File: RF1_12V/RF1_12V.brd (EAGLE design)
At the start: 6.9 x 7.1 mm, 17 parts, among them IC1 L78L33ACZ, IC2 MCP1702, J1 12V, Q1 16mhz, U1 ATMEGA328P_PDIP

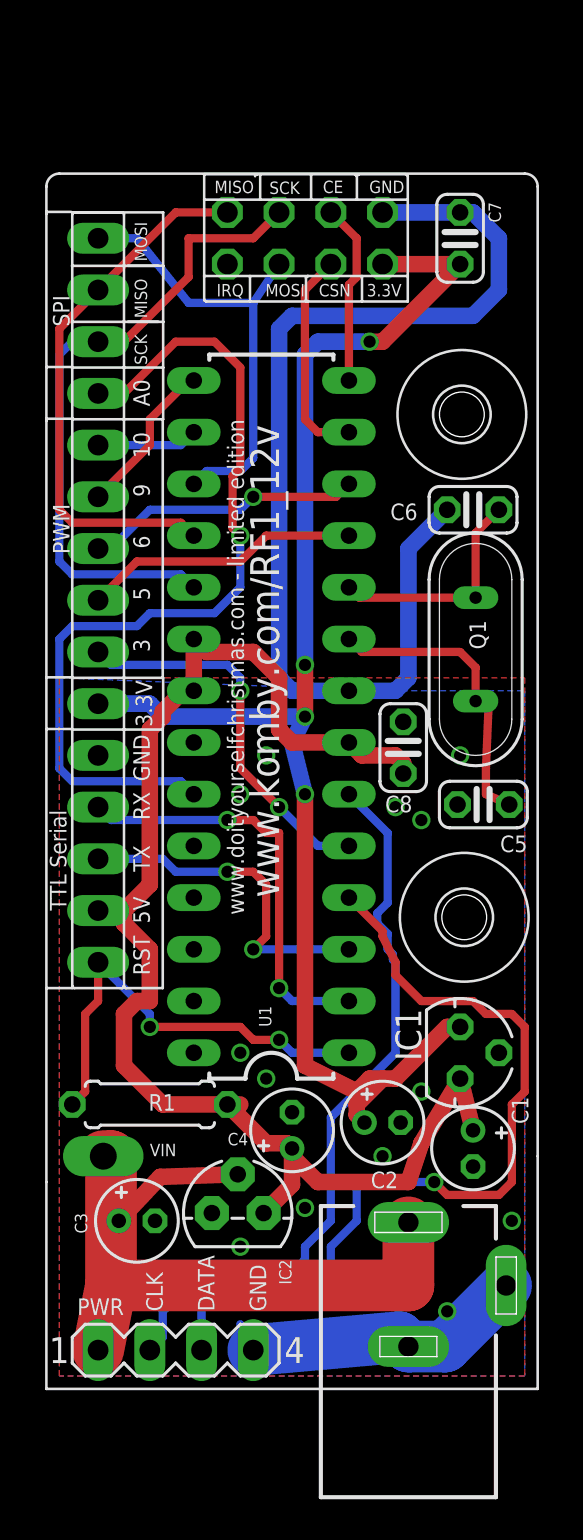
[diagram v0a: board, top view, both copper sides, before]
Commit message: Updated with 2014 designs for both RF1_12v and RF1 5v
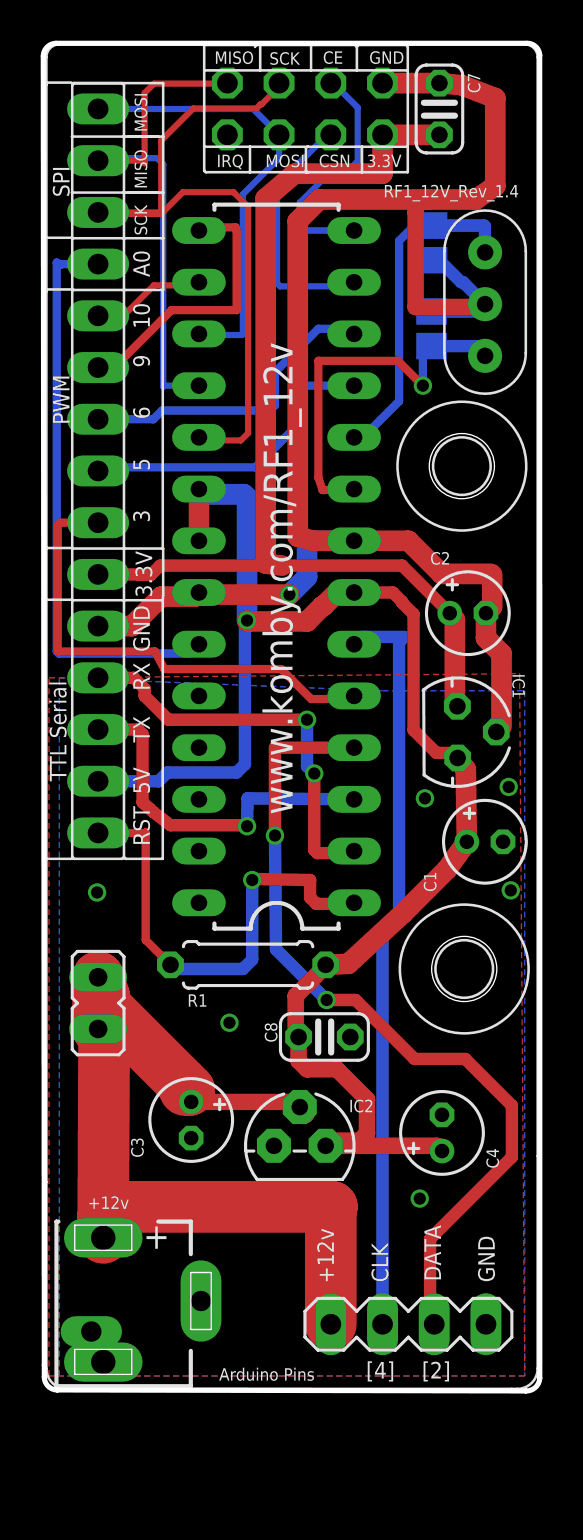
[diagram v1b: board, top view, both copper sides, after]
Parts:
- removed Q1: 16mhz, special:QS
- removed TP1: PTR1PAD1-13Y, testpad:P1-13Y
- added JP1: +12v, jumper:JP1
- added U$2: (no value), adafruit:CERM_OSC
- C2: value .1uf -> .1uF
- C3, C4: value 1uF -> 10uF
- C5, C6: device resistor:C025-024X044 -> adafruit:C0805
- C7, C8: value 100n -> .1uF
- J1: device con-jack:DCJ0303 -> con-jack_komby:DCJ0303
- moved C2 25.4 mm to (20.7, 38.1)
- moved C5 23.5 mm to (18.9, 52.1), flipped to the bottom, turned to 90 degrees
- moved IC1 15.7 mm to (20.2, 32.3), turned to 270.3 degrees
- moved C1 15.1 mm to (21.5, 26.9), turned to 0 degrees
- moved J1 15.0 mm to (2.79, 4.32)
- moved C8 14.7 mm to (13.7, 17.3), turned to 0 degrees
- moved C6 13.3 mm to (18.9, 56.3), flipped to the bottom, turned to 270 degrees
- moved SV1 11.5 mm to (17.8, 3.17)
- moved R1 8.39 mm to (9.91, 20.8)
- moved U1 7.37 mm to (11.3, 40.4)
- moved C4 7.37 mm to (19.4, 12.6)
- moved C7 6.43 mm to (19.3, 62.9)
- moved C3 5.63 mm to (7.11, 13.2), turned to 270 degrees
- moved IC2 4.49 mm to (12.4, 11.9)
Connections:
- net GND: now also U$2.P$2
- net N$5: now also U$2.P$3; no longer Q1.2
- net N$6: now also U$2.P$1; no longer Q1.1
- net VIN: now also JP1.1, JP1.2; no longer TP1.TP
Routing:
- net GND: track 68.7 -> 87.8 mm, vias 13 -> 7
- net 3.3V: track 70.9 -> 52.8 mm, vias 4 -> 0
- net PC0: track 43.2 -> 28.4 mm, vias 1 -> 0
- net VIN: track 39.8 -> 47.9 mm
- net +5V: track 70.0 -> 77.0 mm, vias 0 -> 1
- net PWM4_PB1: track 7.81 -> 13.9 mm
- net N$5: track 11.2 -> 16.7 mm
- net PWM1_PD3: track 18.9 -> 24.0 mm, vias 2 -> 0
- net N$6: track 14.7 -> 18.5 mm, vias 0 -> 1
- net SCK: track 32.1 -> 35.6 mm
- net RF_CE: track 8.94 -> 12.1 mm
- net RESET: track 22.0 -> 24.1 mm, vias 2 -> 1
- net RF_CSN: track 10.6 -> 12.4 mm
- net PWM3_PD6: track 13.6 -> 15.5 mm, vias 1 -> 0
- net PWM2_PD5: track 13.6 -> 15.2 mm
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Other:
- board size 6.9 x 7.1 mm -> 24.4 x 66.2 mm
- board text added: "+12v"
- board text added: "Arduino Pins"
- board text added: "RF1_12V_Rev_1.4"
- board text added: "[2]"
- board text added: "[4]"
- board text removed: "DIYC Edition"
- board text removed: "PWR"
- board text removed: "VIN"
- board text removed: "www.doityourselfchristmas.com - limited edition"
